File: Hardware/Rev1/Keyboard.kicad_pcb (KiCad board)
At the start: 2 copper layers, 129 parts, among them P1 USB_OTG, Q1 IRLML6402, Q10 BSS84, Q11 BSS138, Q12 BSS138, Q13 BSS138, Q14 BSS138, Q15 BSS138, Q2 IRLML6402, Q3 BSS84, Q4 BSS138, Q5 BSS138, Q6 BSS138, Q7 BSS84, Q8 BSS84, Q9 BSS84, SW1 ISP, SW10 SW_PUSH, SW11 SW_PUSH, SW12 SW_PUSH, SW13 SW_PUSH, SW14 SW_PUSH, SW15 SW_PUSH, SW16 SW_PUSH, SW17 SW_PUSH, SW18 SW_PUSH, SW19 SW_PUSH, SW2 SW_PUSH, SW20 SW_PUSH, SW21 SW_PUSH, SW22 SW_PUSH, SW23 SW_PUSH, SW24 SW_PUSH, SW25 SW_PUSH, SW26 SW_PUSH, SW27 SW_PUSH, SW28 SW_PUSH, SW29 SW_PUSH, SW3 SW_PUSH, SW30 SW_PUSH, SW31 SW_PUSH, SW32 SW_PUSH, SW4 SW_PUSH, SW5 SW_PUSH, SW6 SW_PUSH, SW7 SW_PUSH, SW8 SW_PUSH, SW9 SW_PUSH, U1 LPC11U35FHI33/501_DAPLINK, U2 ADP3338AKCZ-3.3, U3 HRM1026, X1 12MHz

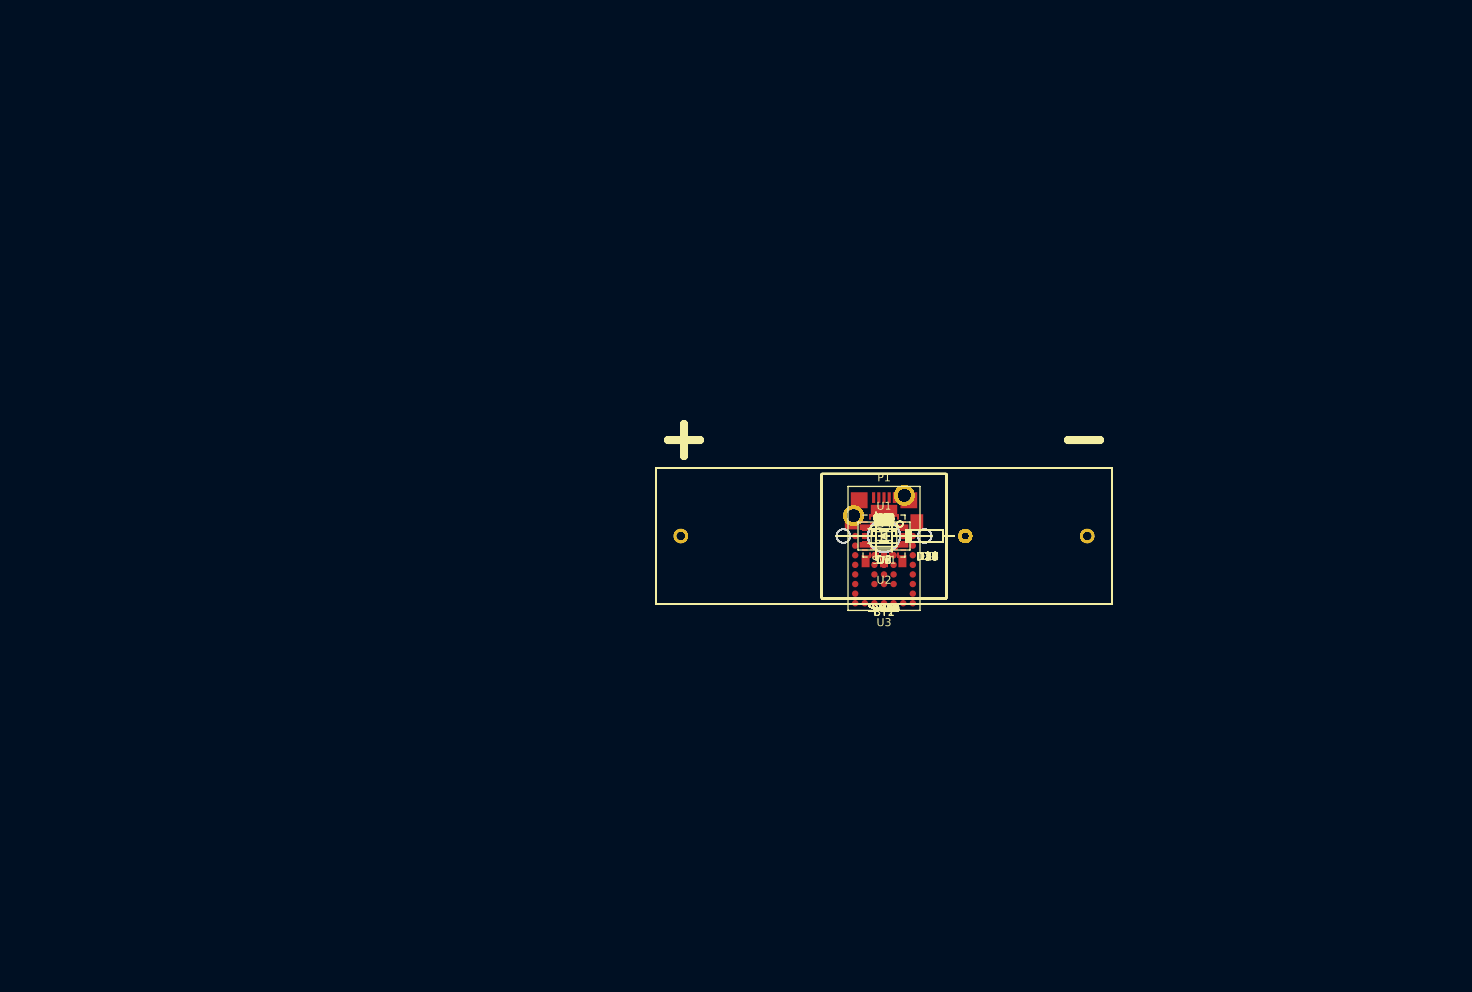
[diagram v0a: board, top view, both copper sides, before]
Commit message: Add Rev1 Left PCB Pattern
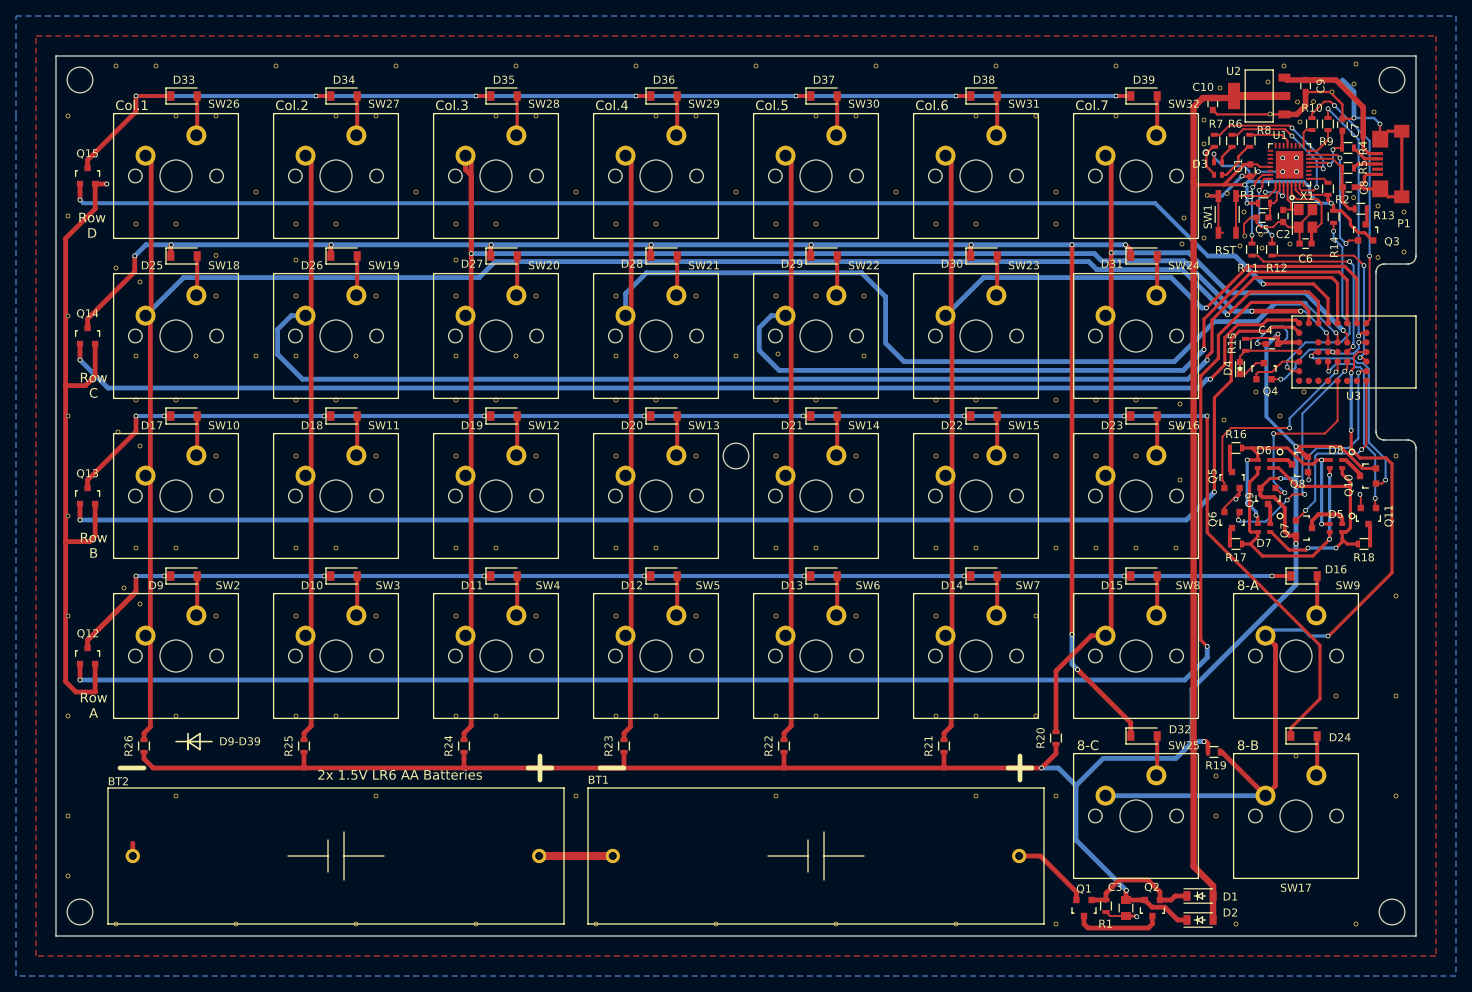
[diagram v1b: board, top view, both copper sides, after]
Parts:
- added REF**: 0.4-0.6_via, guri-lib:0.4-0.6_via, F.Cu at (188.9, 62.4)
- added REF**: 0.4-0.6_via, guri-lib:0.4-0.6_via, F.Cu at (212.5, 137.5)
- added REF**: 0.4-0.6_via, guri-lib:0.4-0.6_via, F.Cu at (82.5, 82.5)
- added REF**: 0.4-0.6_via, guri-lib:0.4-0.6_via, F.Cu at (95.0, 82.5)
- added REF**: 0.4-0.6_via, guri-lib:0.4-0.6_via, F.Cu at (102.5, 82.5)
- added REF**: 0.4-0.6_via, guri-lib:0.4-0.6_via, F.Cu at (115.0, 82.5)
- added REF**: 0.4-0.6_via, guri-lib:0.4-0.6_via, F.Cu at (122.5, 82.5)
- added REF**: 0.4-0.6_via, guri-lib:0.4-0.6_via, F.Cu at (135.2, 82.2)
- added REF**: 0.4-0.6_via, guri-lib:0.4-0.6_via, F.Cu at (130.0, 82.5)
- added REF**: 0.4-0.6_via, guri-lib:0.4-0.6_via, F.Cu at (146.0, 82.5)
- added REF**: 0.4-0.6_via, guri-lib:0.4-0.6_via, F.Cu at (146.0, 75.0)
- added REF**: 0.4-0.6_via, guri-lib:0.4-0.6_via, F.Cu at (140.0, 75.0)
- added REF**: 0.4-0.6_via, guri-lib:0.4-0.6_via, F.Cu at (200.0, 132.5)
- added REF**: 0.4-0.6_via, guri-lib:0.4-0.6_via, F.Cu at (135.0, 75.0)
- added REF**: 0.4-0.6_via, guri-lib:0.4-0.6_via, F.Cu at (125.0, 75.0)
- added REF**: 0.4-0.6_via, guri-lib:0.4-0.6_via, F.Cu at (115.0, 75.0)
- added REF**: 0.4-0.6_via, guri-lib:0.4-0.6_via, F.Cu at (105.0, 75.0)
- added REF**: 0.4-0.6_via, guri-lib:0.4-0.6_via, F.Cu at (95.0, 75.0)
- added REF**: 0.4-0.6_via, guri-lib:0.4-0.6_via, F.Cu at (85.0, 75.0)
- added REF**: 0.4-0.6_via, guri-lib:0.4-0.6_via, F.Cu at (75.0, 75.0)
- added REF**: 0.4-0.6_via, guri-lib:0.4-0.6_via, F.Cu at (65.0, 75.0)
- added REF**: 0.4-0.6_via, guri-lib:0.4-0.6_via, F.Cu at (95.0, 70.5)
- added REF**: 0.4-0.6_via, guri-lib:0.4-0.6_via, F.Cu at (65.0, 70.0)
- added REF**: 0.4-0.6_via, guri-lib:0.4-0.6_via, F.Cu at (205.0, 125.0)
- added REF**: 0.4-0.6_via, guri-lib:0.4-0.6_via, F.Cu at (75.0, 70.5)
- added REF**: 0.4-0.6_via, guri-lib:0.4-0.6_via, F.Cu at (55.0, 66.0)
- added REF**: 0.4-0.6_via, guri-lib:0.4-0.6_via, F.Cu at (60.0, 66.0)
- added REF**: 0.4-0.6_via, guri-lib:0.4-0.6_via, F.Cu at (75.0, 66.0)
- added REF**: 0.4-0.6_via, guri-lib:0.4-0.6_via, F.Cu at (80.0, 66.0)
- added REF**: 0.4-0.6_via, guri-lib:0.4-0.6_via, F.Cu at (95.0, 66.0)
- added REF**: 0.4-0.6_via, guri-lib:0.4-0.6_via, F.Cu at (100.0, 66.0)
- added REF**: 0.4-0.6_via, guri-lib:0.4-0.6_via, F.Cu at (115.0, 66.0)
- added REF**: 0.4-0.6_via, guri-lib:0.4-0.6_via, F.Cu at (120.0, 66.0)
- added REF**: 0.4-0.6_via, guri-lib:0.4-0.6_via, F.Cu at (135.0, 66.0)
- added REF**: 0.4-0.6_via, guri-lib:0.4-0.6_via, F.Cu at (190.0, 140.0)
- added REF**: 0.4-0.6_via, guri-lib:0.4-0.6_via, F.Cu at (140.0, 66.0)
- added REF**: 0.4-0.6_via, guri-lib:0.4-0.6_via, F.Cu at (155.0, 66.0)
- added REF**: 0.4-0.6_via, guri-lib:0.4-0.6_via, F.Cu at (160.0, 66.0)
- added REF**: 0.4-0.6_via, guri-lib:0.4-0.6_via, F.Cu at (170.0, 66.0)
- added REF**: 0.4-0.6_via, guri-lib:0.4-0.6_via, F.Cu at (170.0, 62.0)
- added REF**: 0.4-0.6_via, guri-lib:0.4-0.6_via, F.Cu at (150.0, 62.0)
- added REF**: 0.4-0.6_via, guri-lib:0.4-0.6_via, F.Cu at (130.0, 62.0)
- added REF**: 0.4-0.6_via, guri-lib:0.4-0.6_via, F.Cu at (110.0, 62.0)
- added REF**: 0.4-0.6_via, guri-lib:0.4-0.6_via, F.Cu at (90.0, 62.0)
- added REF**: 0.4-0.6_via, guri-lib:0.4-0.6_via, F.Cu at (70.0, 62.0)
- added REF**: 0.4-0.6_via, guri-lib:0.4-0.6_via, F.Cu at (190.0, 135.0)
- added REF**: 0.4-0.6_via, guri-lib:0.4-0.6_via, F.Cu at (60.0, 52.5)
- added REF**: 0.4-0.6_via, guri-lib:0.4-0.6_via, F.Cu at (65.0, 52.5)
- added REF**: 0.4-0.6_via, guri-lib:0.4-0.6_via, F.Cu at (80.0, 52.5)
- added REF**: 0.4-0.6_via, guri-lib:0.4-0.6_via, F.Cu at (85.0, 52.5)
- added REF**: 0.4-0.6_via, guri-lib:0.4-0.6_via, F.Cu at (100.0, 52.5)
- added REF**: 0.4-0.6_via, guri-lib:0.4-0.6_via, F.Cu at (105.0, 52.5)
- added REF**: 0.4-0.6_via, guri-lib:0.4-0.6_via, F.Cu at (120.0, 52.5)
- added REF**: 0.4-0.6_via, guri-lib:0.4-0.6_via, F.Cu at (125.0, 52.5)
- added REF**: 0.4-0.6_via, guri-lib:0.4-0.6_via, F.Cu at (140.0, 52.5)
- added REF**: 0.4-0.6_via, guri-lib:0.4-0.6_via, F.Cu at (145.0, 52.5)
- added REF**: 0.4-0.6_via, guri-lib:0.4-0.6_via, F.Cu at (170.0, 137.5)
- added REF**: 0.4-0.6_via, guri-lib:0.4-0.6_via, F.Cu at (160.0, 52.5)
- added REF**: 0.4-0.6_via, guri-lib:0.4-0.6_via, F.Cu at (167.5, 52.5)
- added REF**: 0.4-0.6_via, guri-lib:0.4-0.6_via, F.Cu at (177.5, 52.5)
- added REF**: 0.4-0.6_via, guri-lib:0.4-0.6_via, F.Cu at (185.5, 98.0)
- added REF**: 0.4-0.6_via, guri-lib:0.4-0.6_via, F.Cu at (185.5, 91.5)
- added REF**: 0.4-0.6_via, guri-lib:0.4-0.6_via, F.Cu at (185.5, 88.5)
- added REF**: 0.4-0.6_via, guri-lib:0.4-0.6_via, F.Cu at (201.0, 87.0)
- added REF**: 0.4-0.6_via, guri-lib:0.4-0.6_via, F.Cu at (198.0, 90.0)
- added REF**: 0.4-0.6_via, guri-lib:0.4-0.6_via, F.Cu at (195.0, 87.0)
- added REF**: 0.4-0.6_via, guri-lib:0.4-0.6_via, F.Cu at (191.0, 90.5)
- added REF**: 0.4-0.6_via, guri-lib:0.4-0.6_via, F.Cu at (160.0, 137.5)
- added REF**: 0.4-0.6_via, guri-lib:0.4-0.6_via, F.Cu at (207.5, 153.5)
- added REF**: 0.4-0.6_via, guri-lib:0.4-0.6_via, F.Cu at (192.5, 153.5)
- added REF**: 0.4-0.6_via, guri-lib:0.4-0.6_via, F.Cu at (170.0, 153.5)
- added REF**: 0.4-0.6_via, guri-lib:0.4-0.6_via, F.Cu at (157.5, 153.5)
- added REF**: 0.4-0.6_via, guri-lib:0.4-0.6_via, F.Cu at (142.5, 153.5)
- added REF**: 0.4-0.6_via, guri-lib:0.4-0.6_via, F.Cu at (127.5, 153.5)
- added REF**: 0.4-0.6_via, guri-lib:0.4-0.6_via, F.Cu at (112.5, 153.5)
- added REF**: 0.4-0.6_via, guri-lib:0.4-0.6_via, F.Cu at (97.5, 153.5)
- added REF**: 0.4-0.6_via, guri-lib:0.4-0.6_via, F.Cu at (82.5, 153.5)
- added REF**: 0.4-0.6_via, guri-lib:0.4-0.6_via, F.Cu at (67.5, 153.5)
- added REF**: 0.4-0.6_via, guri-lib:0.4-0.6_via, F.Cu at (135.0, 137.5)
- added REF**: 0.4-0.6_via, guri-lib:0.4-0.6_via, F.Cu at (52.5, 153.5)
- added REF**: 0.4-0.6_via, guri-lib:0.4-0.6_via, F.Cu at (46.5, 147.5)
- added REF**: 0.4-0.6_via, guri-lib:0.4-0.6_via, F.Cu at (46.5, 140.0)
- added REF**: 0.4-0.6_via, guri-lib:0.4-0.6_via, F.Cu at (46.5, 127.5)
- added REF**: 0.4-0.6_via, guri-lib:0.4-0.6_via, F.Cu at (46.5, 115.0)
- added REF**: 0.4-0.6_via, guri-lib:0.4-0.6_via, F.Cu at (46.5, 102.5)
- added REF**: 0.4-0.6_via, guri-lib:0.4-0.6_via, F.Cu at (46.5, 90.0)
- added REF**: 0.4-0.6_via, guri-lib:0.4-0.6_via, F.Cu at (46.5, 77.5)
- added REF**: 0.4-0.6_via, guri-lib:0.4-0.6_via, F.Cu at (46.5, 65.0)
- added REF**: 0.4-0.6_via, guri-lib:0.4-0.6_via, F.Cu at (46.5, 52.5)
- added REF**: 0.4-0.6_via, guri-lib:0.4-0.6_via, F.Cu at (110.0, 137.5)
- added REF**: 0.4-0.6_via, guri-lib:0.4-0.6_via, F.Cu at (52.5, 46.2)
- added REF**: 0.4-0.6_via, guri-lib:0.4-0.6_via, F.Cu at (57.5, 46.2)
- added REF**: 0.4-0.6_via, guri-lib:0.4-0.6_via, F.Cu at (72.5, 46.2)
- added REF**: 0.4-0.6_via, guri-lib:0.4-0.6_via, F.Cu at (87.5, 46.2)
- added REF**: 0.4-0.6_via, guri-lib:0.4-0.6_via, F.Cu at (102.5, 46.2)
- added REF**: 0.4-0.6_via, guri-lib:0.4-0.6_via, F.Cu at (117.5, 46.2)
- added REF**: 0.4-0.6_via, guri-lib:0.4-0.6_via, F.Cu at (132.5, 46.2)
- added REF**: 0.4-0.6_via, guri-lib:0.4-0.6_via, F.Cu at (147.5, 46.2)
- added REF**: 0.4-0.6_via, guri-lib:0.4-0.6_via, F.Cu at (162.5, 46.2)
- added REF**: 0.4-0.6_via, guri-lib:0.4-0.6_via, F.Cu at (177.5, 46.2)
- added REF**: 0.4-0.6_via, guri-lib:0.4-0.6_via, F.Cu at (85.0, 137.5)
- added REF**: 0.4-0.6_via, guri-lib:0.4-0.6_via, F.Cu at (190.5, 49.0)
- added REF**: 0.4-0.6_via, guri-lib:0.4-0.6_via, F.Cu at (196.5, 48.2)
- added REF**: 0.4-0.6_via, guri-lib:0.4-0.6_via, F.Cu at (198.5, 46.2)
- added REF**: 0.4-0.6_via, guri-lib:0.4-0.6_via, F.Cu at (207.5, 46.0)
- added REF**: 0.4-0.6_via, guri-lib:0.4-0.6_via, F.Cu at (209.8, 52.0)
- added REF**: 0.4-0.6_via, guri-lib:0.4-0.6_via, F.Cu at (207.2, 48.5)
- added REF**: 0.4-0.6_via, guri-lib:0.4-0.6_via, F.Cu at (200.2, 50.8)
- added REF**: 0.4-0.6_via, guri-lib:0.4-0.6_via, F.Cu at (204.5, 49.5)
- added REF**: 0.4-0.6_via, guri-lib:0.4-0.6_via, F.Cu at (200.5, 53.2)
- added REF**: 0.4-0.6_via, guri-lib:0.4-0.6_via, F.Cu at (196.8, 52.2)
- added REF**: 0.4-0.6_via, guri-lib:0.4-0.6_via, F.Cu at (202.2, 50.7)
- added REF**: 0.4-0.6_via, guri-lib:0.4-0.6_via, F.Cu at (60.0, 137.5)
- added REF**: 0.4-0.6_via, guri-lib:0.4-0.6_via, F.Cu at (188.5, 53.0)
- added REF**: 0.4-0.6_via, guri-lib:0.4-0.6_via, F.Cu at (188.5, 56.0)
- added REF**: 0.4-0.6_via, guri-lib:0.4-0.6_via, F.Cu at (191.4, 62.2)
- added REF**: 0.4-0.6_via, guri-lib:0.4-0.6_via, F.Cu at (185.8, 68.5)
- added REF**: 0.4-0.6_via, guri-lib:0.4-0.6_via, F.Cu at (186.0, 65.2)
- added REF**: 0.4-0.6_via, guri-lib:0.4-0.6_via, F.Cu at (188.5, 67.8)
- added REF**: 0.4-0.6_via, guri-lib:0.4-0.6_via, F.Cu at (193.0, 68.8)
- added REF**: 0.4-0.6_via, guri-lib:0.4-0.6_via, F.Cu at (195.8, 69.0)
- added REF**: 0.4-0.6_via, guri-lib:0.4-0.6_via, F.Cu at (199.2, 68.5)
- added REF**: 0.4-0.6_via, guri-lib:0.4-0.6_via, F.Cu at (210.2, 70.2)
- added REF**: 0.4-0.6_via, guri-lib:0.4-0.6_via, F.Cu at (60.0, 127.5)
- added REF**: 0.4-0.6_via, guri-lib:0.4-0.6_via, F.Cu at (210.2, 63.8)
- added REF**: 0.4-0.6_via, guri-lib:0.4-0.6_via, F.Cu at (213.5, 64.5)
- added REF**: MountingHole_3.2mm_M3, Mounting_Holes:MountingHole_3.2mm_M3, F.Cu at (130.0, 95.0)
- added REF**: MountingHole_3.2mm_M3, Mounting_Holes:MountingHole_3.2mm_M3, F.Cu at (48.0, 48.0)
- added REF**: MountingHole_3.2mm_M3, Mounting_Holes:MountingHole_3.2mm_M3, F.Cu at (48.0, 152.0)
- added REF**: MountingHole_3.2mm_M3, Mounting_Holes:MountingHole_3.2mm_M3, F.Cu at (212.0, 152.0)
- added REF**: MountingHole_3.2mm_M3, Mounting_Holes:MountingHole_3.2mm_M3, F.Cu at (212.0, 48.0)
- added REF**: 0.4-0.6_via, guri-lib:0.4-0.6_via, F.Cu at (213.5, 69.5)
- added REF**: 0.4-0.6_via, guri-lib:0.4-0.6_via, F.Cu at (75.0, 127.5)
- added REF**: 0.4-0.6_via, guri-lib:0.4-0.6_via, F.Cu at (80.0, 127.5)
- added REF**: 0.4-0.6_via, guri-lib:0.4-0.6_via, F.Cu at (95.0, 127.5)
- added REF**: 0.4-0.6_via, guri-lib:0.4-0.6_via, F.Cu at (100.0, 127.5)
- added REF**: 0.4-0.6_via, guri-lib:0.4-0.6_via, F.Cu at (115.0, 127.5)
- added REF**: 0.4-0.6_via, guri-lib:0.4-0.6_via, F.Cu at (120.0, 127.5)
- added REF**: 0.4-0.6_via, guri-lib:0.4-0.6_via, F.Cu at (135.0, 127.5)
- added REF**: 0.4-0.6_via, guri-lib:0.4-0.6_via, F.Cu at (140.0, 127.5)
- added REF**: 0.4-0.6_via, guri-lib:0.4-0.6_via, F.Cu at (195.6, 67.3)
- added REF**: 0.4-0.6_via, guri-lib:0.4-0.6_via, F.Cu at (155.0, 127.5)
- added REF**: 0.4-0.6_via, guri-lib:0.4-0.6_via, F.Cu at (160.0, 127.5)
- added REF**: 0.4-0.6_via, guri-lib:0.4-0.6_via, F.Cu at (167.5, 127.5)
- added REF**: 0.4-0.6_via, guri-lib:0.4-0.6_via, F.Cu at (167.5, 115.0)
- added REF**: 0.4-0.6_via, guri-lib:0.4-0.6_via, F.Cu at (155.0, 115.0)
- added REF**: 0.4-0.6_via, guri-lib:0.4-0.6_via, F.Cu at (145.0, 115.0)
- added REF**: 0.4-0.6_via, guri-lib:0.4-0.6_via, F.Cu at (135.0, 115.0)
- added REF**: 0.4-0.6_via, guri-lib:0.4-0.6_via, F.Cu at (125.0, 115.0)
- added REF**: 0.4-0.6_via, guri-lib:0.4-0.6_via, F.Cu at (115.0, 115.0)
- added REF**: 0.4-0.6_via, guri-lib:0.4-0.6_via, F.Cu at (105.0, 115.0)
- added REF**: 0.4-0.6_via, guri-lib:0.4-0.6_via, F.Cu at (193.5, 64.5)
- added REF**: 0.4-0.6_via, guri-lib:0.4-0.6_via, F.Cu at (95.0, 115.0)
- added REF**: 0.4-0.6_via, guri-lib:0.4-0.6_via, F.Cu at (85.0, 115.0)
- added REF**: 0.4-0.6_via, guri-lib:0.4-0.6_via, F.Cu at (75.0, 115.0)
- added REF**: 0.4-0.6_via, guri-lib:0.4-0.6_via, F.Cu at (65.0, 115.0)
- added REF**: 0.4-0.6_via, guri-lib:0.4-0.6_via, F.Cu at (55.5, 113.5)
- added REF**: 0.4-0.6_via, guri-lib:0.4-0.6_via, F.Cu at (53.5, 111.5)
- added REF**: 0.4-0.6_via, guri-lib:0.4-0.6_via, F.Cu at (55.0, 106.5)
- added REF**: 0.4-0.6_via, guri-lib:0.4-0.6_via, F.Cu at (60.0, 106.5)
- added REF**: 0.4-0.6_via, guri-lib:0.4-0.6_via, F.Cu at (75.0, 106.5)
- added REF**: 0.4-0.6_via, guri-lib:0.4-0.6_via, F.Cu at (80.0, 106.5)
- added REF**: 0.4-0.6_via, guri-lib:0.4-0.6_via, F.Cu at (193.6, 67.5)
- added REF**: 0.4-0.6_via, guri-lib:0.4-0.6_via, F.Cu at (95.0, 106.5)
- added REF**: 0.4-0.6_via, guri-lib:0.4-0.6_via, F.Cu at (100.0, 106.5)
- added REF**: 0.4-0.6_via, guri-lib:0.4-0.6_via, F.Cu at (115.0, 106.5)
- added REF**: 0.4-0.6_via, guri-lib:0.4-0.6_via, F.Cu at (120.0, 106.5)
- added REF**: 0.4-0.6_via, guri-lib:0.4-0.6_via, F.Cu at (135.0, 106.5)
- added REF**: 0.4-0.6_via, guri-lib:0.4-0.6_via, F.Cu at (140.0, 106.5)
- added REF**: 0.4-0.6_via, guri-lib:0.4-0.6_via, F.Cu at (155.0, 106.5)
- added REF**: 0.4-0.6_via, guri-lib:0.4-0.6_via, F.Cu at (160.0, 106.5)
- added REF**: 0.4-0.6_via, guri-lib:0.4-0.6_via, F.Cu at (170.0, 106.5)
- added REF**: 0.4-0.6_via, guri-lib:0.4-0.6_via, F.Cu at (175.0, 106.5)
- added REF**: 0.4-0.6_via, guri-lib:0.4-0.6_via, F.Cu at (207.2, 62.7)
- added REF**: 0.4-0.6_via, guri-lib:0.4-0.6_via, F.Cu at (180.0, 106.5)
- added REF**: 0.4-0.6_via, guri-lib:0.4-0.6_via, F.Cu at (185.0, 106.5)
- added REF**: 0.4-0.6_via, guri-lib:0.4-0.6_via, F.Cu at (175.0, 88.0)
- added REF**: 0.4-0.6_via, guri-lib:0.4-0.6_via, F.Cu at (180.0, 95.0)
- added REF**: 0.4-0.6_via, guri-lib:0.4-0.6_via, F.Cu at (175.0, 95.0)
- added REF**: 0.4-0.6_via, guri-lib:0.4-0.6_via, F.Cu at (170.0, 95.0)
- added REF**: 0.4-0.6_via, guri-lib:0.4-0.6_via, F.Cu at (165.0, 95.0)
- added REF**: 0.4-0.6_via, guri-lib:0.4-0.6_via, F.Cu at (160.0, 95.0)
- added REF**: 0.4-0.6_via, guri-lib:0.4-0.6_via, F.Cu at (155.0, 95.0)
- added REF**: 0.4-0.6_via, guri-lib:0.4-0.6_via, F.Cu at (145.0, 95.0)
- added REF**: 0.4-0.6_via, guri-lib:0.4-0.6_via, F.Cu at (212.5, 95.0)
- added REF**: 0.4-0.6_via, guri-lib:0.4-0.6_via, F.Cu at (135.0, 95.0)
- added REF**: 0.4-0.6_via, guri-lib:0.4-0.6_via, F.Cu at (125.0, 95.0)
- added REF**: 0.4-0.6_via, guri-lib:0.4-0.6_via, F.Cu at (115.0, 95.0)
- added REF**: 0.4-0.6_via, guri-lib:0.4-0.6_via, F.Cu at (105.0, 95.0)
- added REF**: 0.4-0.6_via, guri-lib:0.4-0.6_via, F.Cu at (95.0, 95.0)
- added REF**: 0.4-0.6_via, guri-lib:0.4-0.6_via, F.Cu at (85.0, 95.0)
- added REF**: 0.4-0.6_via, guri-lib:0.4-0.6_via, F.Cu at (75.0, 95.0)
- added REF**: 0.4-0.6_via, guri-lib:0.4-0.6_via, F.Cu at (65.0, 95.0)
- added REF**: 0.4-0.6_via, guri-lib:0.4-0.6_via, F.Cu at (52.8, 92.0)
- added REF**: 0.4-0.6_via, guri-lib:0.4-0.6_via, F.Cu at (55.5, 93.8)
- added REF**: 0.4-0.6_via, guri-lib:0.4-0.6_via, F.Cu at (212.5, 112.5)
- added REF**: 0.4-0.6_via, guri-lib:0.4-0.6_via, F.Cu at (52.5, 71.5)
- added REF**: 0.4-0.6_via, guri-lib:0.4-0.6_via, F.Cu at (55.5, 73.2)
- added REF**: 0.4-0.6_via, guri-lib:0.4-0.6_via, F.Cu at (180.0, 88.0)
- added REF**: 0.4-0.6_via, guri-lib:0.4-0.6_via, F.Cu at (170.0, 88.0)
- added REF**: 0.4-0.6_via, guri-lib:0.4-0.6_via, F.Cu at (160.0, 88.0)
- added REF**: 0.4-0.6_via, guri-lib:0.4-0.6_via, F.Cu at (155.0, 88.0)
- added REF**: 0.4-0.6_via, guri-lib:0.4-0.6_via, F.Cu at (140.0, 88.0)
- added REF**: 0.4-0.6_via, guri-lib:0.4-0.6_via, F.Cu at (135.0, 88.0)
- added REF**: 0.4-0.6_via, guri-lib:0.4-0.6_via, F.Cu at (120.0, 88.0)
- added REF**: 0.4-0.6_via, guri-lib:0.4-0.6_via, F.Cu at (115.0, 88.0)
- added REF**: 0.4-0.6_via, guri-lib:0.4-0.6_via, F.Cu at (212.5, 125.0)
- added REF**: 0.4-0.6_via, guri-lib:0.4-0.6_via, F.Cu at (100.0, 88.0)
- added REF**: 0.4-0.6_via, guri-lib:0.4-0.6_via, F.Cu at (95.0, 88.0)
- added REF**: 0.4-0.6_via, guri-lib:0.4-0.6_via, F.Cu at (80.0, 88.0)
- added REF**: 0.4-0.6_via, guri-lib:0.4-0.6_via, F.Cu at (75.0, 88.0)
- added REF**: 0.4-0.6_via, guri-lib:0.4-0.6_via, F.Cu at (60.0, 88.0)
- added REF**: 0.4-0.6_via, guri-lib:0.4-0.6_via, F.Cu at (55.0, 88.0)
- added REF**: 0.4-0.6_via, guri-lib:0.4-0.6_via, F.Cu at (55.0, 82.5)
- added REF**: 0.4-0.6_via, guri-lib:0.4-0.6_via, F.Cu at (62.5, 82.5)
- added REF**: 0.4-0.6_via, guri-lib:0.4-0.6_via, F.Cu at (70.0, 82.5)
- added REF**: 0.4-0.6_via, guri-lib:0.4-0.6_via, F.Cu at (75.0, 82.5)
- D10, D11, D12, D13, D14, D15, D16, D17, D18, D19, D20, D21, D22, D23, D24, D25, D26, D27, D28, D29, D30, D31, D32, D33, D34, D35, D36, D37, D38, D39, D9: footprint Diodes_ThroughHole:Diode_DO-35_SOD27_Horizontal_RM10 -> Diodes_SMD:D_SOD-123
- X1: footprint Crystals:crystal_FA238-TSX3225 -> Crystals:Crystal_SMD_3225-4pin_3.2x2.5mm
- moved Q15 109.3 mm to (49.0, 60.0)
- moved D33 103.4 mm to (61.0, 50.0)
- moved Q14 102.6 mm to (49.0, 80.0)
- moved Q12 100.7 mm to (49.0, 120.0)
- moved Q13 99.7 mm to (49.0, 100.0)
- moved SW26 99.3 mm to (60.0, 60.0)
- moved R26 96.2 mm to (56.0, 131.2), turned to 90 degrees
- moved D25 94.2 mm to (61.0, 70.0)
- moved SW18 92.0 mm to (60.0, 80.0)
- moved SW2 89.8 mm to (60.0, 120.0)
- moved D17 88.8 mm to (61.0, 90.0)
- moved SW10 88.6 mm to (60.0, 100.0)
- moved D9 87.6 mm to (61.0, 110.0)
- moved D34 87.1 mm to (81.0, 50.0)
- moved SW27 82.0 mm to (80.0, 60.0)
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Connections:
- net Col.A renamed RowA
- net Col.B renamed RowB
- net Col.C renamed RowC
- net Col.D renamed RowD
- net Row1 renamed Col.1
- net Row2 renamed Col.2
- net Row3 renamed Col.3
- net Row4 renamed Col.4
- net Row5 renamed Col.5
- net Row6 renamed Col.6
- net Row7 renamed Col.7
- net Row8 renamed Col.8
- C4 pad 1: +3V3 -> VCC
- Q3 pad 2: GND -> +3V3
- R14 pad 1: USB_Detect -> USBDetect
- X1 pad 2: Net-(C6-Pad1) -> GND
- X1 pad 3: GND -> Net-(C6-Pad1)
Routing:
- net VCC: track 0.00 -> 273.1 mm, vias 0 -> 7
- net Col.1: track 0.00 -> 231.8 mm, vias 0 -> 1
- net Col.2: track 0.00 -> 231.2 mm, vias 0 -> 1
- net GND: track 0.00 -> 220.3 mm, vias 0 -> 16
- net Net-(D25-Pad1): track 0.00 -> 210.5 mm, vias 0 -> 11
- net RowA: track 0.00 -> 200.6 mm, vias 0 -> 2
- net Col.3: track 0.00 -> 198.9 mm, vias 0 -> 4
- net Net-(D17-Pad1): track 0.00 -> 198.9 mm, vias 0 -> 9
- net Col.4: track 0.00 -> 181.9 mm, vias 0 -> 1
- net RowB: track 0.00 -> 174.6 mm, vias 0 -> 2
- net Net-(D10-Pad1): track 0.00 -> 170.3 mm, vias 0 -> 9
- net Col.5: track 0.00 -> 169.9 mm, vias 0 -> 1
- net +3V3: track 0.00 -> 166.7 mm, vias 0 -> 4
- net RowD: track 0.00 -> 166.2 mm, vias 0 -> 2
- net RowC: track 0.00 -> 161.5 mm, vias 0 -> 2
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- added copper zone on B.Cu, net GND
- added copper zone on F.Cu, net GND
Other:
- board outline added: 170 x 110 mm
- board text added: "2018/01"
- board text added: "2x 1.5V LR6 AA Batteries"
- board text added: "8-A"
- board text added: "8-B"
- board text added: "8-C"
- board text added: "Col.1"
- board text added: "Col.2"
- board text added: "Col.3"
- board text added: "Col.4"
- board text added: "Col.5"
- board text added: "Col.6"
- board text added: "Col.7"
- board text added: "D9-D39"
- board text added: "Designed By @zgtk-guri"
- board text added: "HOGP Separate Keyboard R1"
- board text added: "RST"
- board text added: "Row A"
- board text added: "Row B"
- board text added: "Row C"
- board text added: "Row D"
- board text added: "for Left hand"
